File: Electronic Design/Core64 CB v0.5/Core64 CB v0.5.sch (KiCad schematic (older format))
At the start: 20 parts, among them J1 Digi-Key 77311-420-36LF-ND, J2 Digi-Key 77311-420-36LF-ND, U1 SI7210-B-01, U2 SI7210-B-02, U3 SI7210-B-03, U4 SI7210-B-04, U5 BH1730FVC

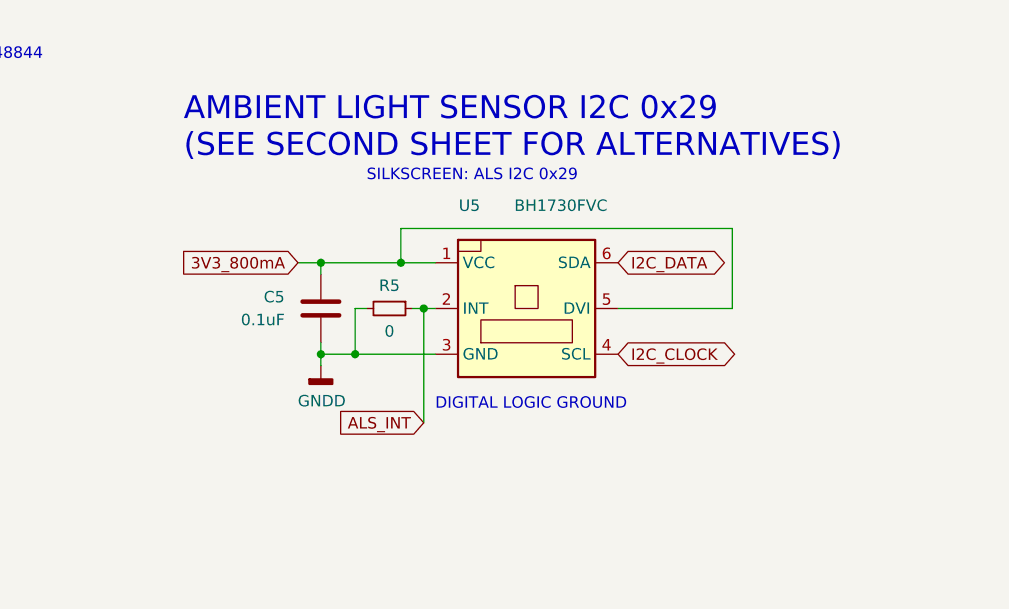
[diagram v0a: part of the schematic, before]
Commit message: Refine and release LB and CB V0.5 layout for prototyping
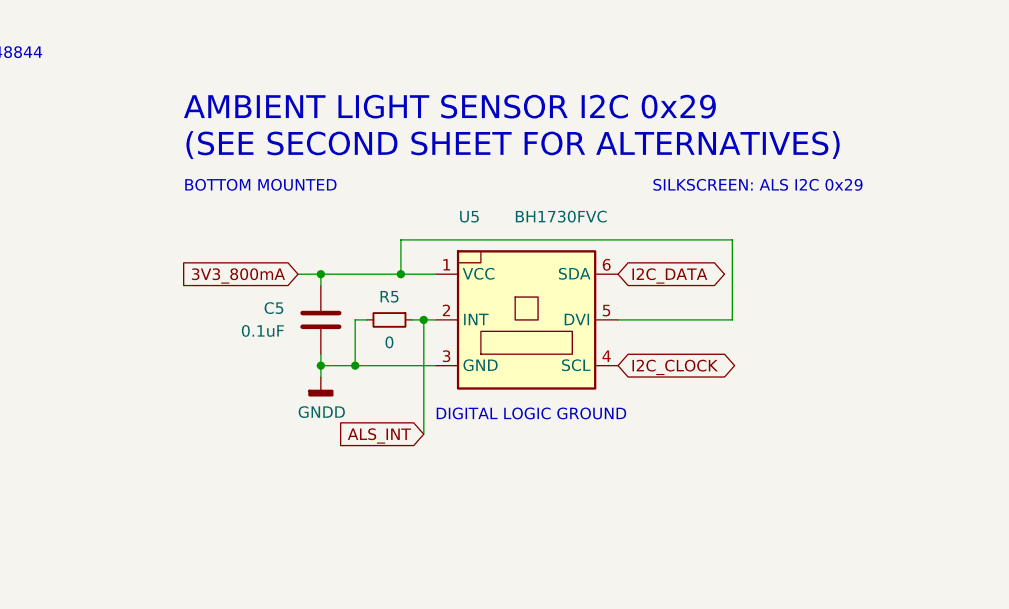
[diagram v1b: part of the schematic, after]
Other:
- note added: "BOTTOM MOUNTED"
- moved on the sheet: C5, R5, U5
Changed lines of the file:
@@
 Sheet 1 2
 Title "Core64 CB (Core Board)"
-Date "2021-02-15"
+Date "2021-02-27"
 Rev "0.5"
 Comp "Concept and design by Andy Geppert @ www.MachineIdeas.com"
@@
 Wire Wire Line
 	8350 3000 8050 3000
-Text Notes 8100 5550 0    50   ~ 0
+Text Notes 9350 5600 0    50   ~ 0
 SILKSCREEN: ALS I2C 0x29
 $Comp
@@
 L Core_64_KiCad_Library:BH1730FVC U5
 U 1 1 604130EC
-P 8800 6100
-F 0 "U5" H 8550 6550 50  0000 C CNN
-F 1 "BH1730FVC" H 8950 6550 50  0000 C CNN
-F 2 "ALS_BH1730:BH1730-backside" H 8800 6550 50  0001 C CNN
-F 3 "http://optoelectronics.liteon.com/upload/download/DS86-2013-0004/LTR-303ALS-01_DS_V1.pdf" H 8500 6450 50  0001 C CNN
-F 4 "C79616" H 8800 6100 50  0001 C CNN "LCSC"
-	1    8800 6100
+P 8800 6150
+F 0 "U5" H 8550 6600 50  0000 C CNN
+F 1 "BH1730FVC" H 8950 6600 50  0000 C CNN
+F 2 "ALS_BH1730:BH1730-backside" H 8800 6600 50  0001 C CNN
+F 3 "http://optoelectronics.liteon.com/upload/download/DS86-2013-0004/LTR-303ALS-01_DS_V1.pdf" H 8500 6500 50  0001 C CNN
+F 4 "C79616" H 8800 6150 50  0001 C CNN "LCSC"
+	1    8800 6150
 	1    0    0    -1
 $EndComp
@@
 L Device:C C5
 U 1 1 60495262
-P 7900 6100
-F 0 "C5" H 7650 6150 50  0000 L CNN
-F 1 "0.1uF" H 7550 6050 50  0000 L CNN
-F 2 "Capacitor_SMD:C_0805_2012Metric" H 7938 5950 50  0001 C CNN
-F 3 "~" H 7900 6100 50  0001 C CNN
-F 4 "C396718" H 7900 6100 50  0001 C CNN "LCSC"
-	1    7900 6100
-	1    0    0    -1
-$EndComp
-Text Notes 8400 6550 0    50   ~ 0
+P 7900 6150
+F 0 "C5" H 7650 6200 50  0000 L CNN
+F 1 "0.1uF" H 7550 6100 50  0000 L CNN
+F 2 "Capacitor_SMD:C_0805_2012Metric" H 7938 6000 50  0001 C CNN
+F 3 "~" H 7900 6150 50  0001 C CNN
+F 4 "C396718" H 7900 6150 50  0001 C CNN "LCSC"
+	1    7900 6150
+	1    0    0    -1
+$EndComp
+Text Notes 8400 6600 0    50   ~ 0
 DIGITAL LOGIC GROUND
 $Comp
 L power:GNDD #PWR01
 U 1 1 60495269
-P 7900 6350
-F 0 "#PWR01" H 7900 6100 50  0001 C CNN
-F 1 "GNDD" H 7904 6195 50  0000 C CNN
-F 2 "" H 7900 6350 50  0001 C CNN
-F 3 "" H 7900 6350 50  0001 C CNN
-	1    7900 6350
-	1    0    0    -1
-$EndComp
-Wire Wire Line
-	7900 6300 8050 6300
-Wire Wire Line
-	7900 6300 7900 6350
-Wire Wire Line
-	7900 5900 7900 5950
-Text GLabel 7800 5900 0    50   Input ~ 0
+P 7900 6400
+F 0 "#PWR01" H 7900 6150 50  0001 C CNN
+F 1 "GNDD" H 7904 6245 50  0000 C CNN
+F 2 "" H 7900 6400 50  0001 C CNN
+F 3 "" H 7900 6400 50  0001 C CNN
+	1    7900 6400
+	1    0    0    -1
+$EndComp
+Wire Wire Line
+	7900 6350 8050 6350
+Wire Wire Line
+	7900 6350 7900 6400
+Wire Wire Line
+	7900 5950 7900 6000
+Text GLabel 7800 5950 0    50   Input ~ 0
 3V3_800mA
-Text GLabel 9200 5900 2    50   BiDi ~ 0
+Text GLabel 9200 5950 2    50   BiDi ~ 0
 I2C_DATA
-Text GLabel 9200 6300 2    50   BiDi ~ 0
+Text GLabel 9200 6350 2    50   BiDi ~ 0
 I2C_CLOCK
 Wire Wire Line
-	7900 5900 7800 5900
-Connection ~ 7900 5900
-Wire Wire Line
-	7900 6300 7900 6250
-Connection ~ 7900 6300
+	7900 5950 7800 5950
+Connection ~ 7900 5950
+Wire Wire Line
+	7900 6350 7900 6300
+Connection ~ 7900 6350
 $Comp
 L Device:R_Small R5
 U 1 1 602E2405
-P 8200 6100
-F 0 "R5" V 8100 6100 50  0000 C CNN
-F 1 "0" V 8300 6100 50  0000 C CNN
-F 2 "Resistor_SMD:R_0805_2012Metric" H 8200 6100 50  0001 C CNN
-F 3 "~" H 8200 6100 50  0001 C CNN
-F 4 "C115306" V 8200 6100 50  0001 C CNN "LCSC"
-	1    8200 6100
+P 8200 6150
+F 0 "R5" V 8100 6150 50  0000 C CNN
+F 1 "0" V 8300 6150 50  0000 C CNN
+F 2 "Resistor_SMD:R_0805_2012Metric" H 8200 6150 50  0001 C CNN
+F 3 "~" H 8200 6150 50  0001 C CNN
+F 4 "C115306" V 8200 6150 50  0001 C CNN "LCSC"
+	1    8200 6150
 	0    1    1    0
 $EndComp
 Wire Wire Line
-	8400 6100 8350 6100
-Wire Wire Line
-	8100 6100 8050 6100
-Wire Wire Line
-	8250 5900 8250 5750
-Wire Wire Line
-	8250 5750 9700 5750
-Wire Wire Line
-	9700 5750 9700 6100
-Connection ~ 8250 5900
-Wire Wire Line
-	8250 5900 8400 5900
-Wire Wire Line
-	9200 6100 9700 6100
-Wire Wire Line
-	7900 5900 8250 5900
-Wire Wire Line
-	8050 6100 8050 6300
-Connection ~ 8050 6300
-Wire Wire Line
-	8050 6300 8400 6300
-Wire Wire Line
-	8350 6100 8350 6600
-Connection ~ 8350 6100
-Wire Wire Line
-	8350 6100 8300 6100
+	8400 6150 8350 6150
+Wire Wire Line
+	8100 6150 8050 6150
+Wire Wire Line
+	8250 5950 8250 5800
+Wire Wire Line
+	8250 5800 9700 5800
+Wire Wire Line
+	9700 5800 9700 6150
+Connection ~ 8250 5950
+Wire Wire Line
+	8250 5950 8400 5950
+Wire Wire Line
+	9200 6150 9700 6150
+Wire Wire Line
+	7900 5950 8250 5950
+Wire Wire Line
+	8050 6150 8050 6350
+Connection ~ 8050 6350
+Wire Wire Line
+	8050 6350 8400 6350
+Wire Wire Line
+	8350 6150 8350 6650
+Connection ~ 8350 6150
+Wire Wire Line
+	8350 6150 8300 6150
 $Sheet
 S 5050 5550 1350 900
@@
 F1 "Core64 CB V0.5 Optional.sch" 50
 $EndSheet
-Text GLabel 8350 6600 0    50   Input ~ 0
+Text GLabel 8350 6650 0    50   Input ~ 0
 ALS_INT
 Wire Notes Line
@@
 Wire Notes Line
 	2150 1100 2150 2250
+Text Notes 7300 5600 0    50   ~ 0
+BOTTOM MOUNTED
 $EndSCHEMATC
